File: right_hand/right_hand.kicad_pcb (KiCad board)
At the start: 2 copper layers, 165 x 110 mm, 87 parts, among them U0 SW_Push

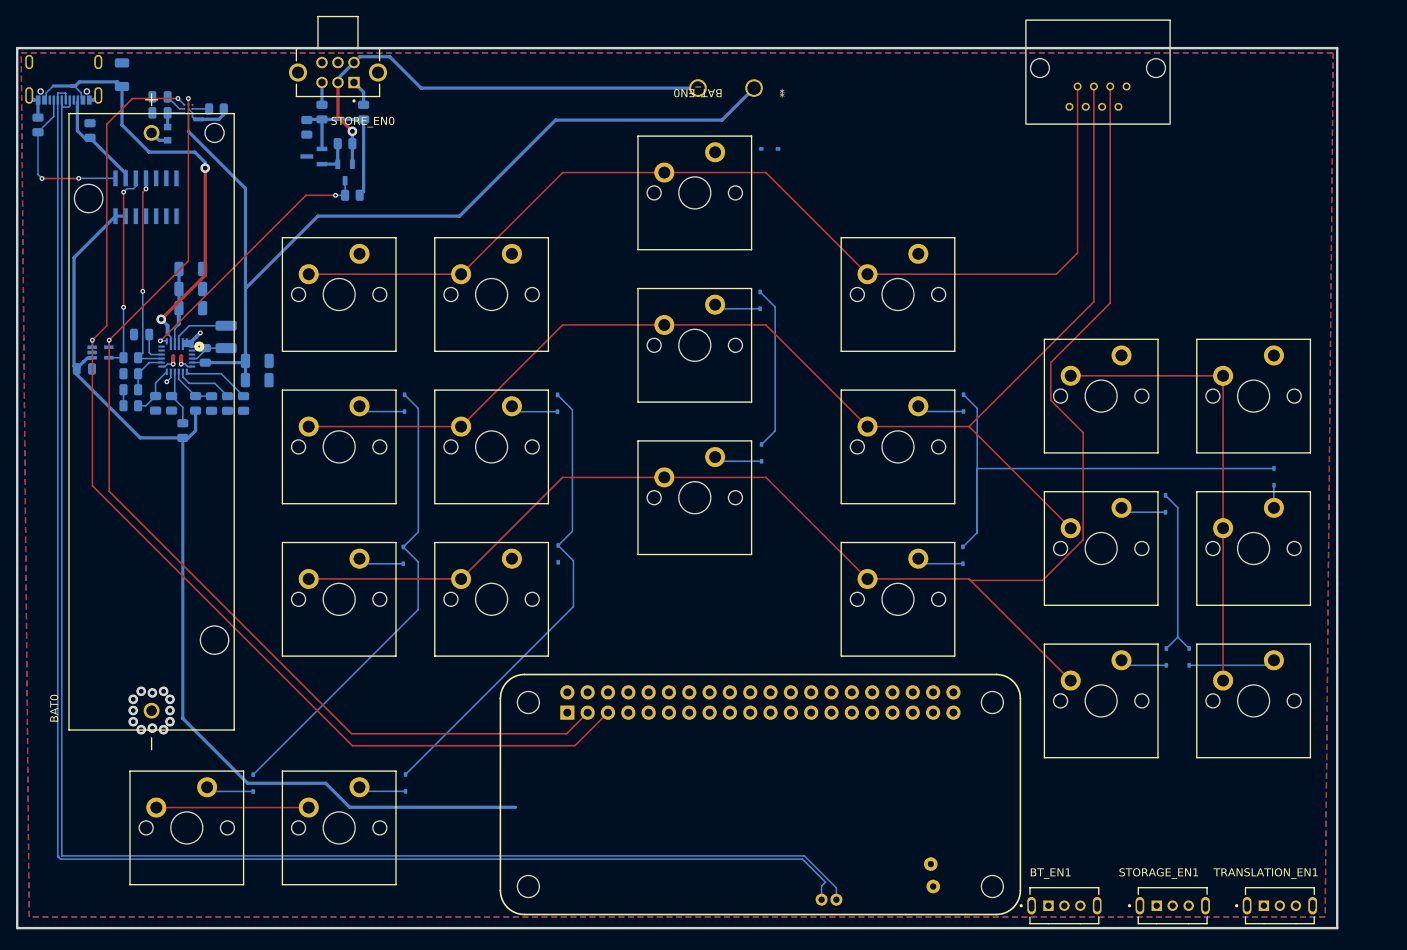
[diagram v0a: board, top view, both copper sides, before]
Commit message: Rework right hand
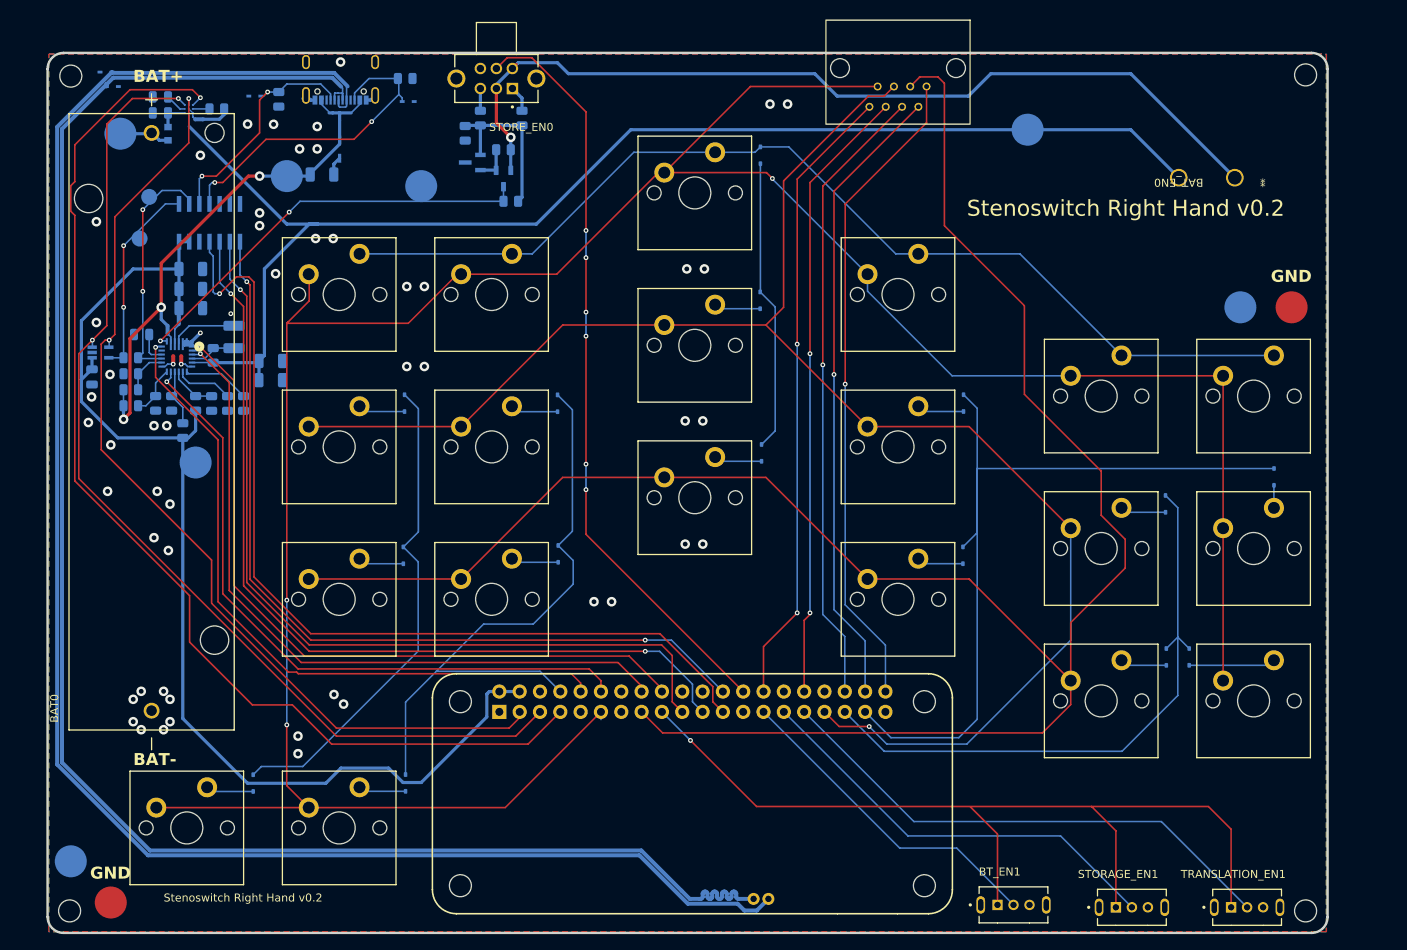
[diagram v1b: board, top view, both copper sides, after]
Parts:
- added ?: , , F.Cu at (87.8, 88.2)
- added ?: , , F.Cu at (226.6, 39.8)
- added ?: , , B.Cu at (224.8, 68.8)
- added ?: , , B.Cu at (78.4, 47.1)
- added ?: , , B.Cu at (77.2, 143.2)
- added ?: , , F.Cu at (218.4, 68.8)
- added ?: , , F.Cu at (226.6, 144.2)
- added ?: , , F.Cu at (99.2, 52.4)
- added ?: , , F.Cu at (116.0, 53.6)
- added ?: , , F.Cu at (72.0, 144.2)
- added ?: , , F.Cu at (72.2, 39.9)
- added ?: , , F.Cu at (82.0, 55.0)
- added ?: , , F.Cu at (72.2, 138.1)
- added CHRG_DIV_{L}: TestPoint_Pad_D2.0mm, TestPoint:TestPoint_Pad_D2.0mm, B.Cu at (80.8, 60.2)
- added CR0: ESD321DYAR, ultra_librarian_footprints:SOT5x3_DYA_TEX, B.Cu at (77.4, 41.2)
- added CR1: ESD321DYAR, ultra_librarian_footprints:SOT5x3_DYA_TEX, B.Cu at (76.6, 39.4)
- added CR2: TSD05DYFR, ultra_librarian_footprints:TVS_SOD2_DYF_TEX, B.Cu at (105.8, 49.0)
- added CR3: ESD321DYAR, ultra_librarian_footprints:SOT5x3_DYA_TEX, B.Cu at (95.2, 42.4)
- added CR4: ESD321DYAR, ultra_librarian_footprints:SOT5x3_DYA_TEX, B.Cu at (114.4, 43.1)
- added REF**: TestPoint_Pad_D4.0mm, TestPoint:TestPoint_Pad_D4.0mm, B.Cu at (191.8, 46.6)
- moved BAT_EN0 61.1 mm to (217.7, 52.6)
- moved USB_Default_Power_CC2 39.9 mm to (114.0, 40.2), turned to 0 degrees
- moved Wired_Interface1 34.6 mm to (105.9, 38.1)
- moved USB_Default_Power_CC1 30.3 mm to (98.2, 42.8), turned to -90 degrees
- moved VBUS_Bypass0 27.9 mm to (103.6, 52.2), turned to 0 degrees
- moved Right_Plug0 25.0 mm to (175.6, 39.4)
- moved BAT_MIN0 19.8 mm to (126.3, 52.7)
- moved R_{Pullup}0 19.8 mm to (126.3, 49.1)
- moved R_{Upper}0 19.8 mm to (123.4, 45.1)
- moved STORE_EN0 19.8 mm to (125.4, 40.2)
- moved R_{HIST}0 19.8 mm to (127.2, 55.5)
- moved R_{Lower}0 19.8 mm to (121.5, 47.0)
- moved R_{Store}0 19.8 mm to (128.6, 45.1)
- moved VBAT_PASS0 19.8 mm to (122.4, 50.7)
- moved Current_Monitor1 8.56 mm to (89.5, 58.2)
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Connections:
- A1 pad 10: unconnected-(A1-GP15/RXD-Pad10) -> /Control/CHG_{EN}
- A1 pad 11: Net-(A1-GP17) -> /Rows2
- A1 pad 12: unconnected-(A1-GP18-Pad12) -> /Control/USB_{ON}
- A1 pad 13: Net-(A1-GP27) -> unconnected-(A1-GP27-Pad13)
- A1 pad 14: unconnected-(A1-GND-Pad14) -> GND
- A1 pad 15: Net-(A1-GP22) -> /Rows1
- A1 pad 16: unconnected-(A1-GP23-Pad16) -> /Control/BAT_{ON}
- A1 pad 17: unconnected-(A1-+3V3-Pad17) -> Net-(A1-+3V3-Pad17)
- A1 pad 18: unconnected-(A1-GP24-Pad18) -> /Control/CHG_{ON}
- A1 pad 2: unconnected-(A1-+5V-Pad2) -> /Control/V_{SYS}
- A1 pad 25: unconnected-(A1-GND-Pad25) -> GND
- A1 pad 26: unconnected-(A1-GP7/CS1-Pad26) -> /Control/STORE_{ON}
- A1 pad 27: unconnected-(A1-GP0-Pad27) -> Net-(A1-GP0)
- A1 pad 28: unconnected-(A1-GP1-Pad28) -> /Left_Columns0
- A1 pad 29: unconnected-(A1-GP5-Pad29) -> Net-(A1-GP5)
- A1 pad 30: unconnected-(A1-GND-Pad30) -> GND
- A1 pad 31: unconnected-(A1-GP6-Pad31) -> Net-(A1-GP6)
- A1 pad 32: unconnected-(A1-GP12/PWM0-Pad32) -> /Left_Columns1
- A1 pad 33: unconnected-(A1-GP13/PWM1-Pad33) -> /Rows0
- A1 pad 34: unconnected-(A1-GND-Pad34) -> GND
- A1 pad 35: unconnected-(A1-GP19-Pad35) -> /Control/Right_Columns0
- A1 pad 36: unconnected-(A1-GP16-Pad36) -> /Left_Columns2
- A1 pad 37: unconnected-(A1-GP26-Pad37) -> /Control/Right_Columns1
- A1 pad 38: unconnected-(A1-GP20-Pad38) -> /Left_Columns3
- A1 pad 4: unconnected-(A1-+5V-Pad4) -> /Control/V_{SYS}
- A1 pad 40: unconnected-(A1-GP21-Pad40) -> /Left_Columns4
- A1 pad 8: unconnected-(A1-GP14/TXD-Pad8) -> /Control/Right_Columns3
- A1 pad 9: unconnected-(A1-GND-Pad9) -> GND
- BAT_EN0 pad 1: Net-(Battery_Charger0-BATT) -> Net-(BAT_EN0-Pad1)
- BAT_EN0 pad 2: Net-(BAT_EN0-Pad2) -> Net-(Battery_Charger0-BATT)
- BAT_MIN0 pad 2: Net-(BAT_EN0-Pad2) -> Net-(BAT_EN0-Pad1)
- BT_EN1 pad 1: /Control/3.3V_Input -> Net-(A1-+3V3-Pad17)
- BT_EN1 pad 2: Net-(A1-GP22) -> Net-(A1-GP0)
- Current_Monitor1 pad 1: Net-(Current_Monitor1-CH0) -> /Interface/Battery/CHRG_DIV_{L}
- Current_Monitor1 pad 2: Net-(Current_Monitor1-CH1) -> /Interface/Battery/CHRG_DIV_{H}
- Current_Monitor1 pad 3: /Interface/Battery/CHRG_DIV_{L} -> Net-(Current_Monitor1-CH2)
- Current_Monitor1 pad 4: /Interface/Battery/CHRG_DIV_{H} -> Net-(Current_Monitor1-CH3)
- R_{Pullup}0 pad 1: Net-(BAT_EN0-Pad2) -> Net-(BAT_EN0-Pad1)
- Right_Plug0 pad 2: /Left_Columns0 -> /Left_Columns2
- Right_Plug0 pad 4: /Left_Columns2 -> /Left_Columns0
- STORAGE_EN1 pad 1: /Control/3.3V_Input -> Net-(A1-+3V3-Pad17)
- STORAGE_EN1 pad 2: Net-(A1-GP27) -> Net-(A1-GP5)
- STORE_EN0 pad 2: Net-(BAT_EN0-Pad2) -> Net-(BAT_EN0-Pad1)
- STORE_EN0 pad 4: Net-(BAT_EN0-Pad2) -> Net-(BAT_EN0-Pad1)
- TRANSLATION_EN1 pad 1: /Control/3.3V_Input -> Net-(A1-+3V3-Pad17)
- TRANSLATION_EN1 pad 2: Net-(A1-GP17) -> Net-(A1-GP6)
- USB_Default_Power_CC1 pad 1: Net-(Current_Monitor1-CH0) -> Net-(Current_Monitor1-CH2)
- USB_Default_Power_CC2 pad 1: Net-(Current_Monitor1-CH1) -> Net-(Current_Monitor1-CH3)
- Wired_Interface1 pad A5: Net-(Current_Monitor1-CH0) -> Net-(Current_Monitor1-CH2)
- Wired_Interface1 pad B5: Net-(Current_Monitor1-CH1) -> Net-(Current_Monitor1-CH3)
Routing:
- net /Control/ALERT_{BATMON}: track 0.00 -> 142.1 mm, vias 0 -> 1
- net /Rows2: track 204.7 -> 336.9 mm, vias 0 -> 3
- net Net-(D_{NUM}1-A): track 0.00 -> 130.6 mm
- net /Control/CLK_{CURRENT}: track 0.00 -> 116.4 mm, vias 0 -> 1
- net Net-(A1-+3V3-Pad17): track 0.00 -> 114.5 mm, vias 0 -> 1
- net Net-(BAT_EN0-Pad1): track 0.00 -> 114.4 mm, vias 0 -> 1
- net /Control/DOUT_{CURRENT}: track 0.00 -> 109.4 mm, vias 0 -> 2
- net /Control/DIN_{CURRENT}: track 0.00 -> 108.0 mm, vias 0 -> 1
- net /Control/CS_{CURRENT}: track 0.00 -> 107.6 mm, vias 0 -> 2
- net /Control/STORE_{ON}: track 0.00 -> 95.2 mm, vias 0 -> 6
- net /Control/CHG_{ON}: track 0.00 -> 92.0 mm, vias 0 -> 1
- net /Control/BAT_{ON}: track 0.00 -> 89.4 mm, vias 0 -> 1
- net /Control/CHG_{EN}: track 0.00 -> 86.4 mm, vias 0 -> 1
- net /Control/USB_{ON}: track 1.46 -> 84.0 mm
- net /Left_Columns4: track 0.00 -> 82.0 mm, vias 0 -> 1
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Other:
- board size 165 x 110 mm -> 160 x 110 mm
- board text added: "*"
- board text added: "BAT+"
- board text added: "BAT-"
- board text added: "CHRG_DIV_{H}"
- board text added: "GND"
- board text added: "MODE"
- board text added: "Stenoswitch Right Hand v0.2"
- board text added: "V_{BAT}"
- board text added: "V_{SYS}"
